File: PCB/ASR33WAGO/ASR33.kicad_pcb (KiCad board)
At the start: 2 copper layers, 70 x 70 mm, 41 parts, among them J1 Tx, J2 Rx, J3 Run, J4 Pwr, J5 Mtr, J6 Reset, J7 USB-C-Socket-V, J8 TC2030-USB-NL-DS, J9 DC, Q1 NX7002AK, SW1 SW_Push, U1 MD8942, U3 NCR402U, U4 NCR402U, U5 LTV-356T, U8 ESP32-S3-MINI-1

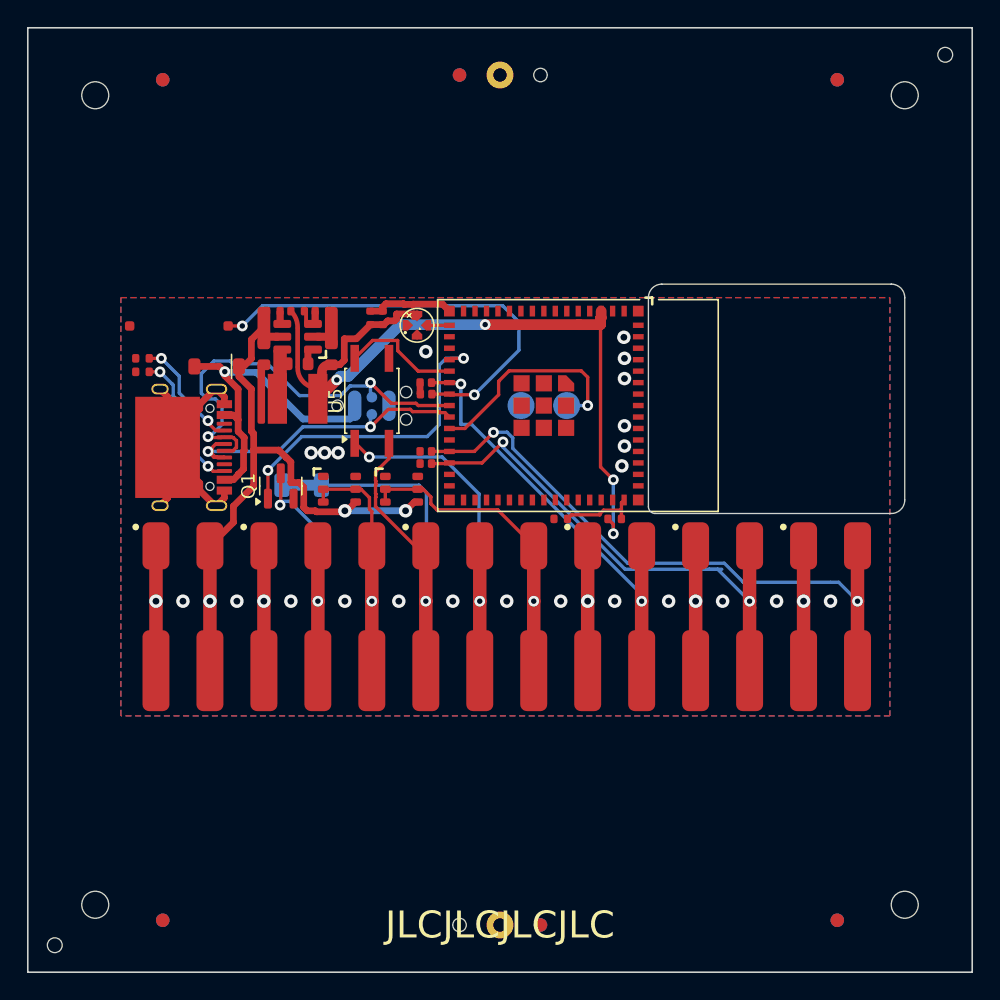
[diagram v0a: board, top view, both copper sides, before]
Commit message: Footprint update
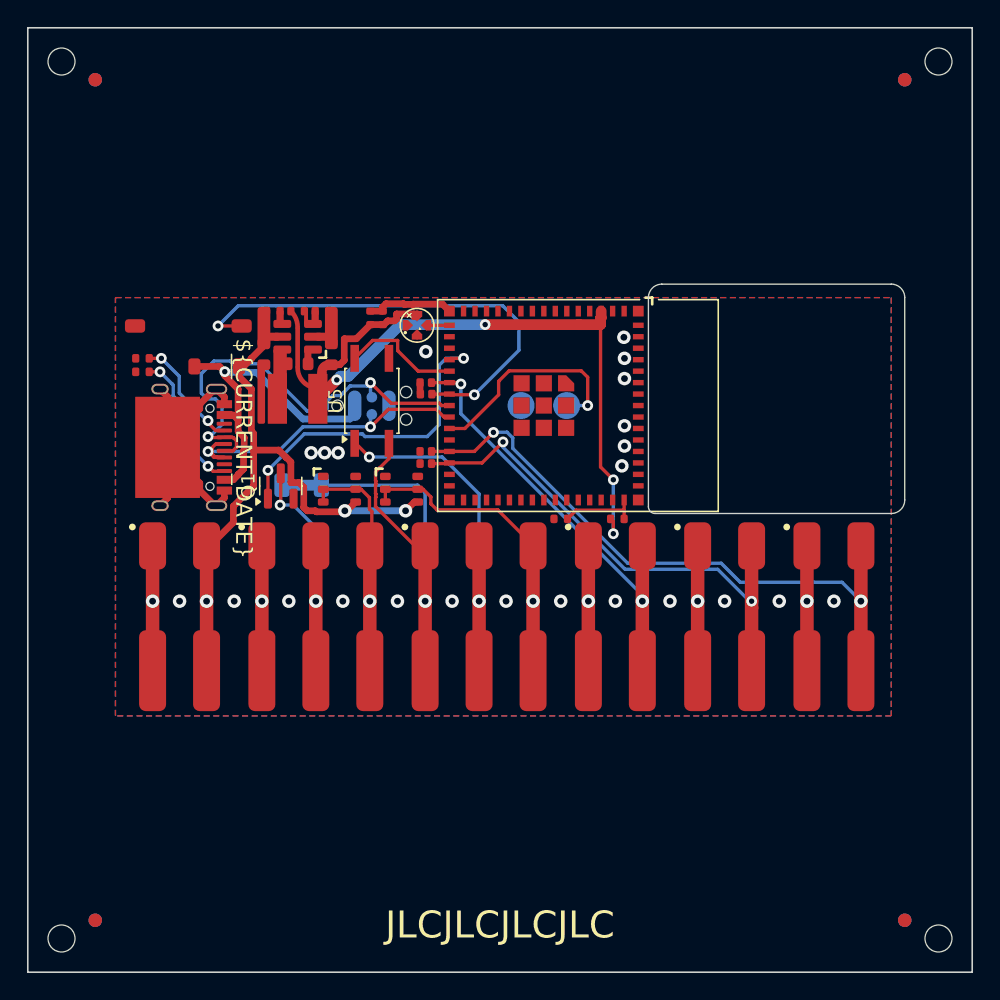
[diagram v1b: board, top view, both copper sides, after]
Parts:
- moved SW1 0.70 mm to (76.9, 87.1)
- moved J5 0.25 mm to (124.8, 108.0)
- moved J9 0.25 mm to (76.2, 108.0)
- moved R13 0.20 mm to (108.7, 101.4)
- moved J1 0.15 mm to (86.3, 108.0)
- moved J4 0.15 mm to (116.7, 108.0)
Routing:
- net BUTTON: track 32.6 -> 35.0 mm
- net DC: track 45.1 -> 43.8 mm
- net D-: track 31.9 -> 32.9 mm
- net PWR: track 39.5 -> 38.5 mm
- net Net-(J2-Pin_1): track 36.0 -> 35.0 mm
- net GND: track 78.0 -> 77.5 mm
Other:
- board text added: "5V-36V"
